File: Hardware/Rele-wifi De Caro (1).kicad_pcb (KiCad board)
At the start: 2 copper layers, 79.3 x 70.1 mm, 38 parts, among them IC1 MC7805CD2TG, J1 Screw_Terminal_01x03, J2 Screw_Terminal_01x03, J3 Screw_Terminal_01x03, J4 Screw_Terminal_01x03, J5 Screw_Terminal_01x02, K1 PR13-5V-450-1C, K2 PR13-5V-450-1C, K3 PR13-5V-450-1C, K4 PR13-5V-450-1C, Q1 PC817-B, Q2 PC817-B, Q3 BC547, Q4 BC547, Q5 PC817-B, Q6 BC547, Q7 PC817-B, Q8 BC547, SW1 SW_DPST_x2, U2 ESP32-CAM

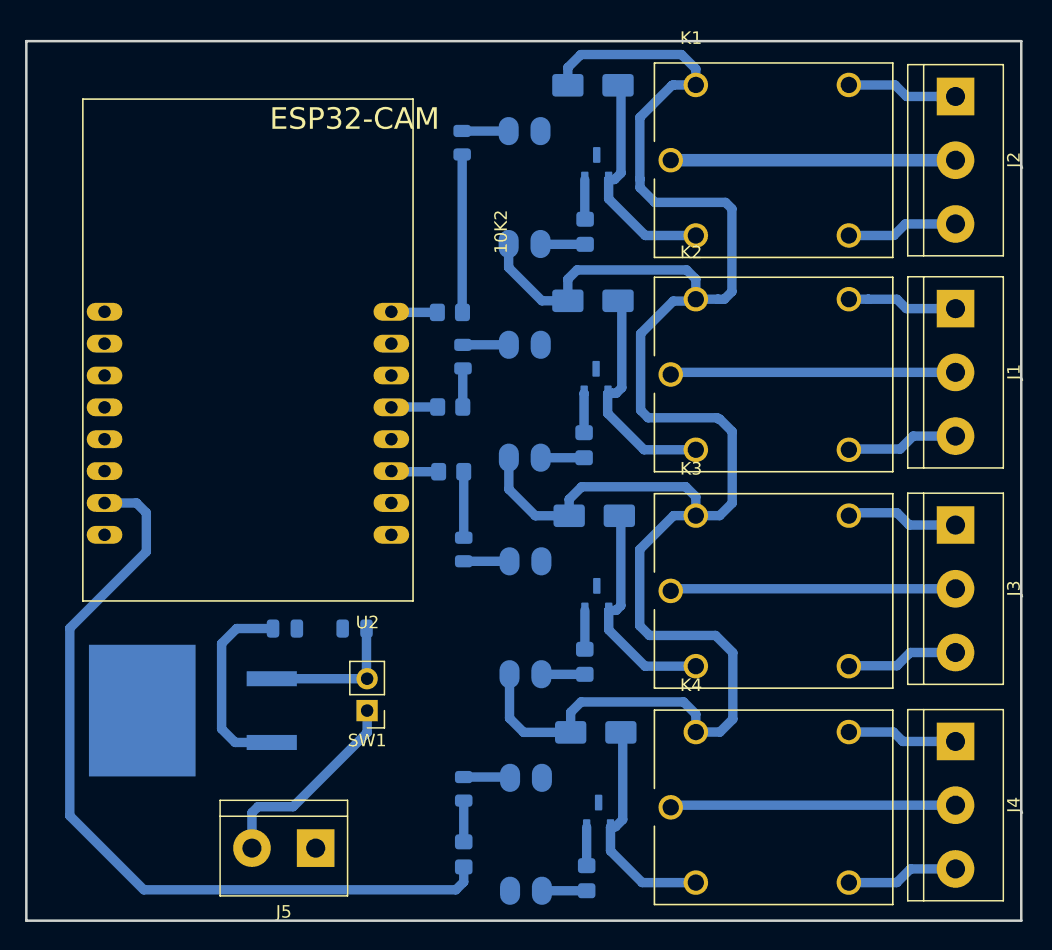
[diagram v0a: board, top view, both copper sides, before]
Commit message: PCB terminado
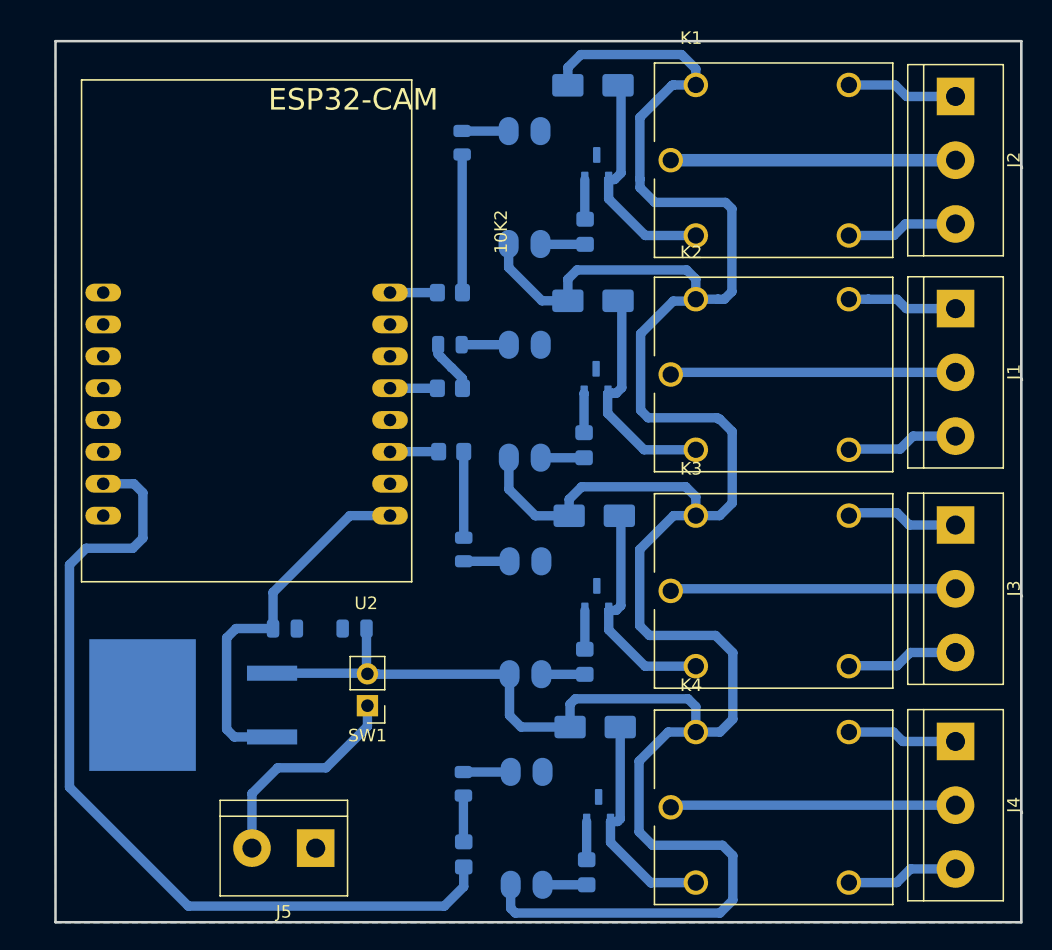
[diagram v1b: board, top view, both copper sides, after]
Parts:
- moved R3 1.60 mm to (160.3, 75.9)
- moved R2 1.57 mm to (160.2, 63.2)
- moved U2 1.53 mm to (144.0, 70.8)
- moved R1 1.49 mm to (160.2, 70.8)
- moved D1 1.41 mm to (160.2, 67.4), turned to 180 degrees
- moved Q7 0.48 mm to (166.3, 105.9)
- moved 10K4 0.48 mm to (171.1, 109.4)
- moved Q8 0.45 mm to (172.1, 104.4)
- moved IC1 0.44 mm to (140.0, 96.1)
- moved D8 0.43 mm to (171.8, 97.8)
- moved D7 0.40 mm to (161.3, 102.4)
- moved SW1 0.39 mm to (153.6, 96.2)
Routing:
- net VCC: track 177.9 -> 232.2 mm
- net Net-(IC1-VOUT): track 15.8 -> 29.9 mm
- net GPIO 16: track 65.6 -> 69.1 mm
- net Net-(D5-A): track 5.26 -> 6.86 mm
- net Net-(D2-A): track 12.6 -> 11.0 mm
- net Net-(D1-A): track 3.08 -> 4.28 mm
- net Net-(J5-Pin_2): track 16.4 -> 17.4 mm
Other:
- board size 79.3 x 70.1 mm -> 77 x 70.2 mm
